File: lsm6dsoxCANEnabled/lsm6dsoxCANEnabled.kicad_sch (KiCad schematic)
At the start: 35 parts, among them J1 CANH and CANL, J2 GPIO, J3 Power, J4 SWD, SW1 Nrst, SW2 BOOT0 selector, U2 TJA1051T, U3 STM32F103C8Tx, U4 AMS1117CD-3.3, Y1 Crystal_GND24

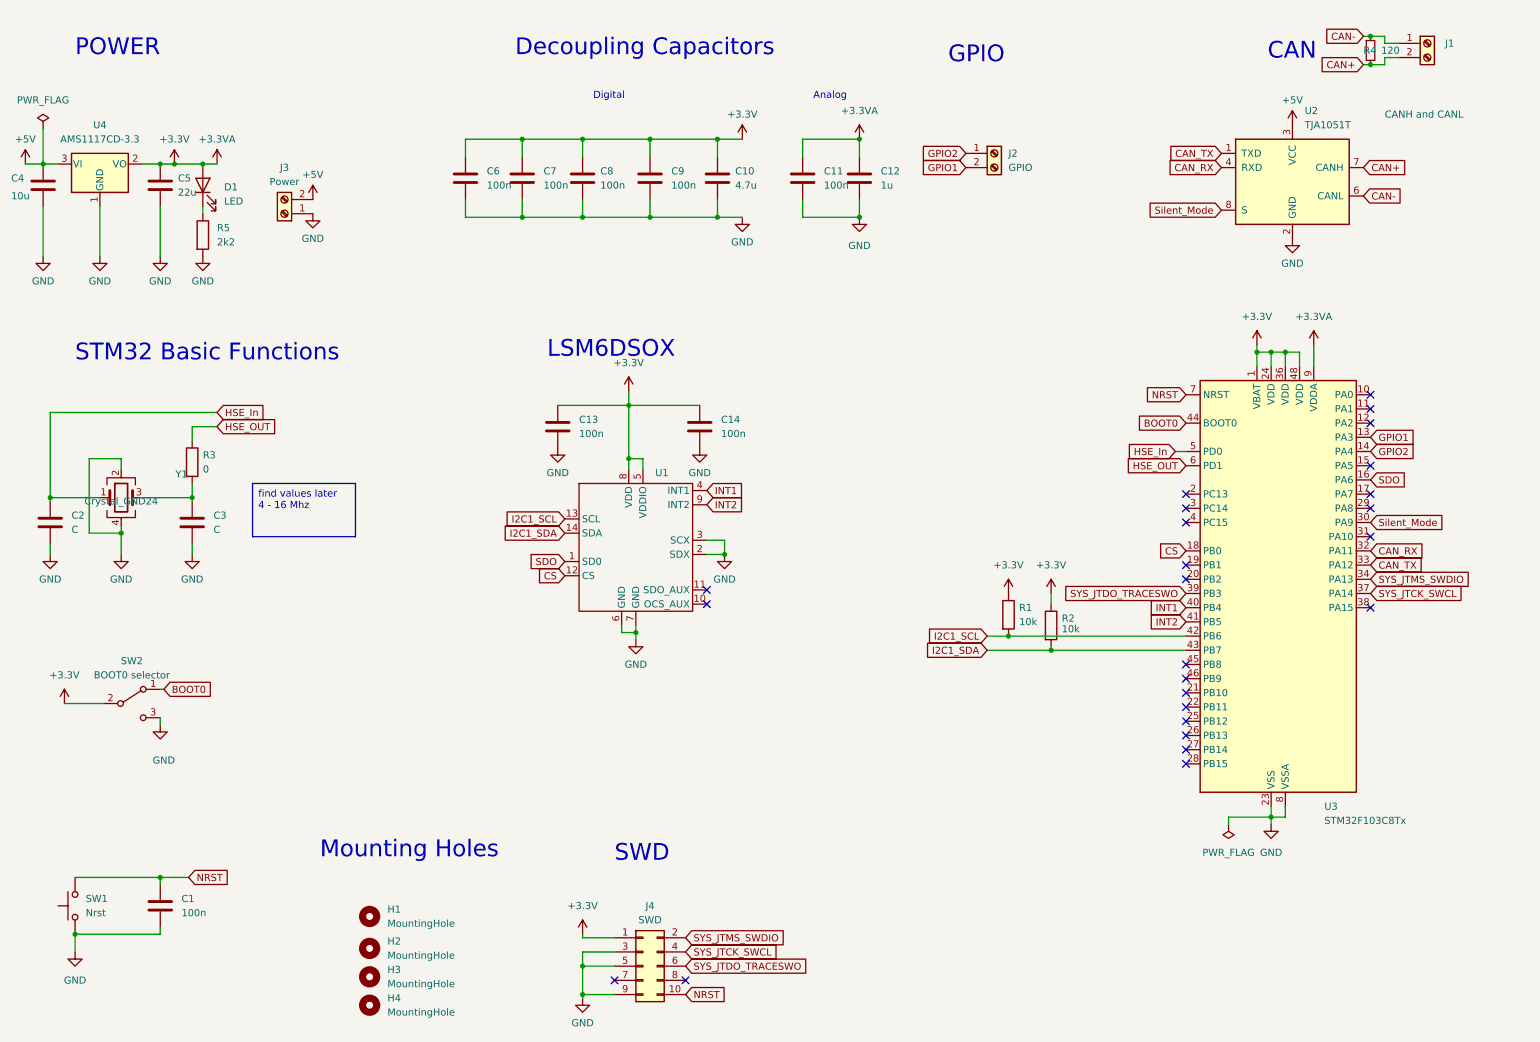
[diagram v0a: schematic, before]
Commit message: updated some stuff
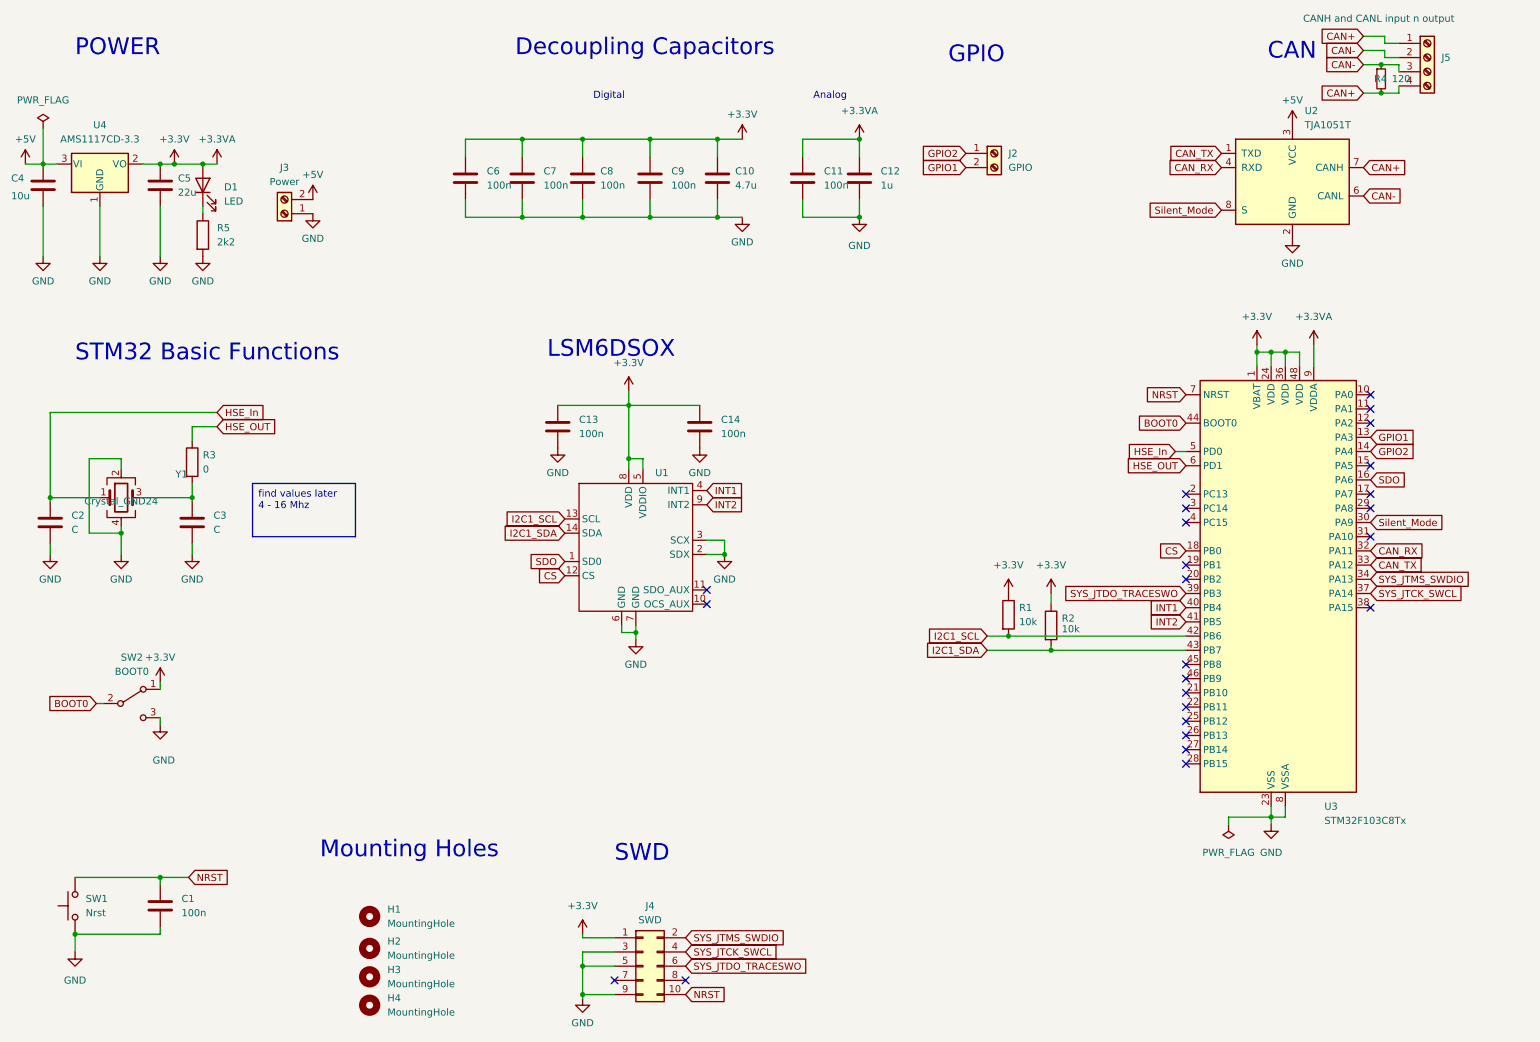
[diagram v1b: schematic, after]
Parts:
- removed J1: CANH and CANL, TerminalBlock_Phoenix:TerminalBlock_Phoenix_MKDS-1,5-2_1x02_P5.00mm_Horizontal, symbol Connector:Screw_Terminal_01x02
- added J5: CANH and CANL input n output, TerminalBlock_Phoenix:TerminalBlock_Phoenix_MKDS-1,5-4_1x04_P5.00mm_Horizontal, symbol Connector:Screw_Terminal_01x04
- SW2: value BOOT0 selector -> BOOT0
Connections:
- net +3.3V: now also SW2.1 (A); no longer SW2.2 (B)
- net BOOT0: now also SW2.2 (B); no longer SW2.1 (A)
- net CAN+: now also J5.1 (Pin_1), J5.4 (Pin_4)
- net CAN-: now also J5.2 (Pin_2), J5.3 (Pin_3)
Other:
- moved on the sheet: R4

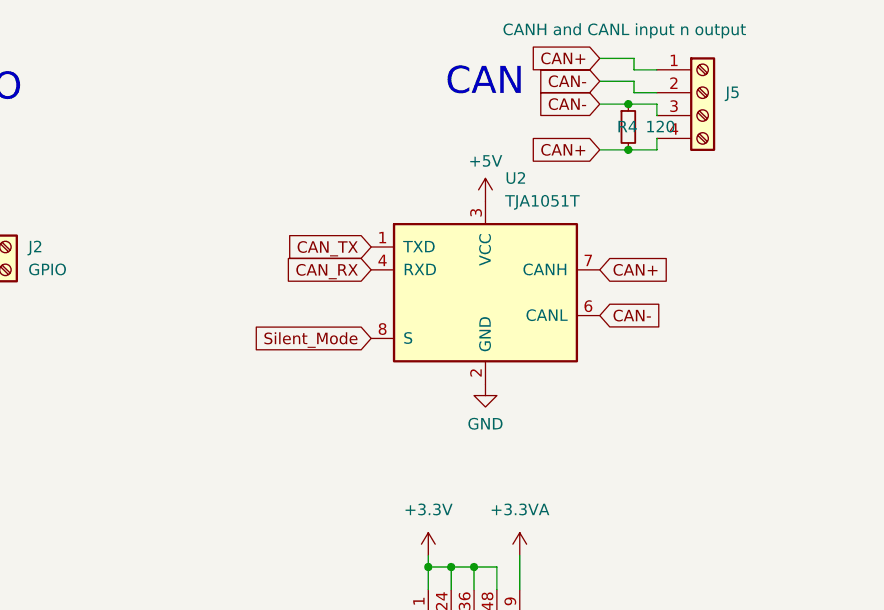
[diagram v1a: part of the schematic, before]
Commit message: added finishing touches to the rev 2 design
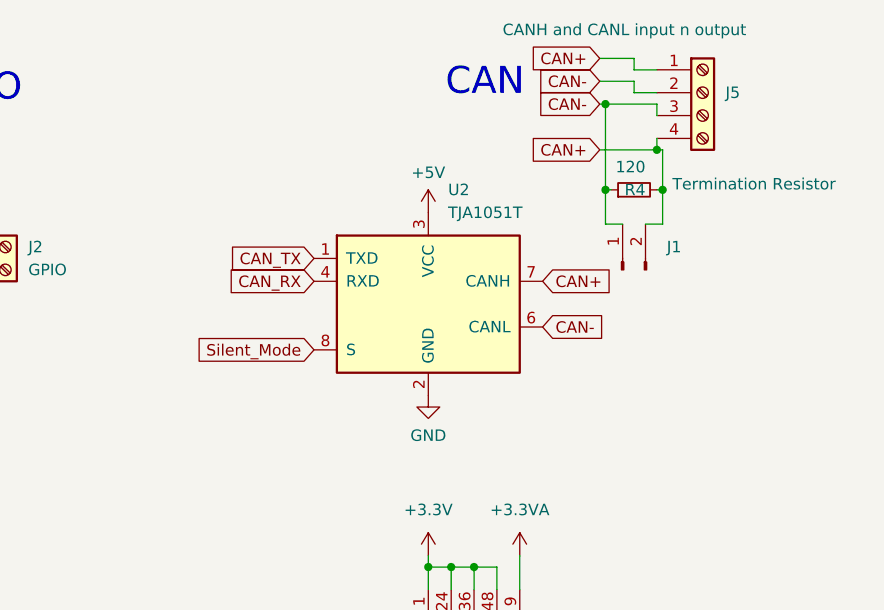
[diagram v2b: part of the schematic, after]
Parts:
- added J1: Termination Resistor, Connector_PinHeader_2.54mm:PinHeader_1x02_P2.54mm_Vertical, symbol Connector:Conn_01x02_Pin
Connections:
- net CAN+: now also J1.2 (Pin_2)
- net CAN-: now also J1.1 (Pin_1)
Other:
- moved on the sheet: R4, U2
